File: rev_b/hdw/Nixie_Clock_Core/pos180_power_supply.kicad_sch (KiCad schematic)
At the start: 27 parts, among them Q601 IRFL214, U1301 TLV6700, U601 LT3757

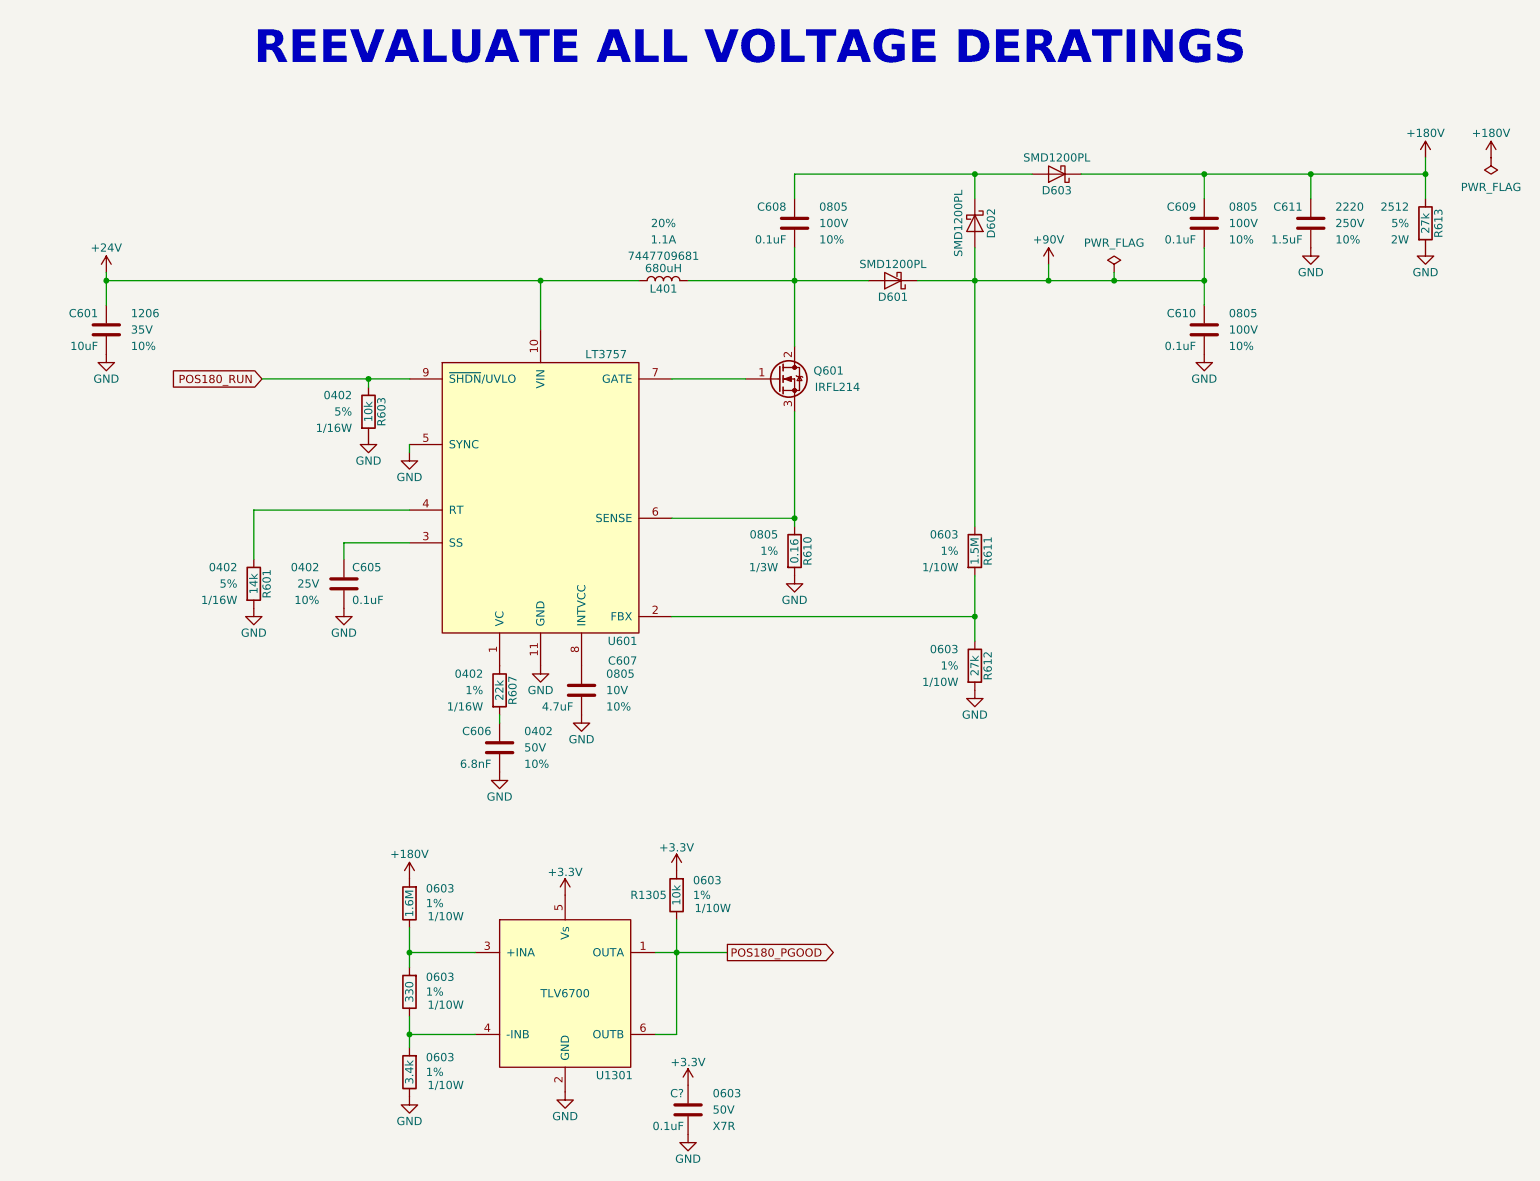
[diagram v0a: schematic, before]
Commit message: lots of rev B control board schematic progress
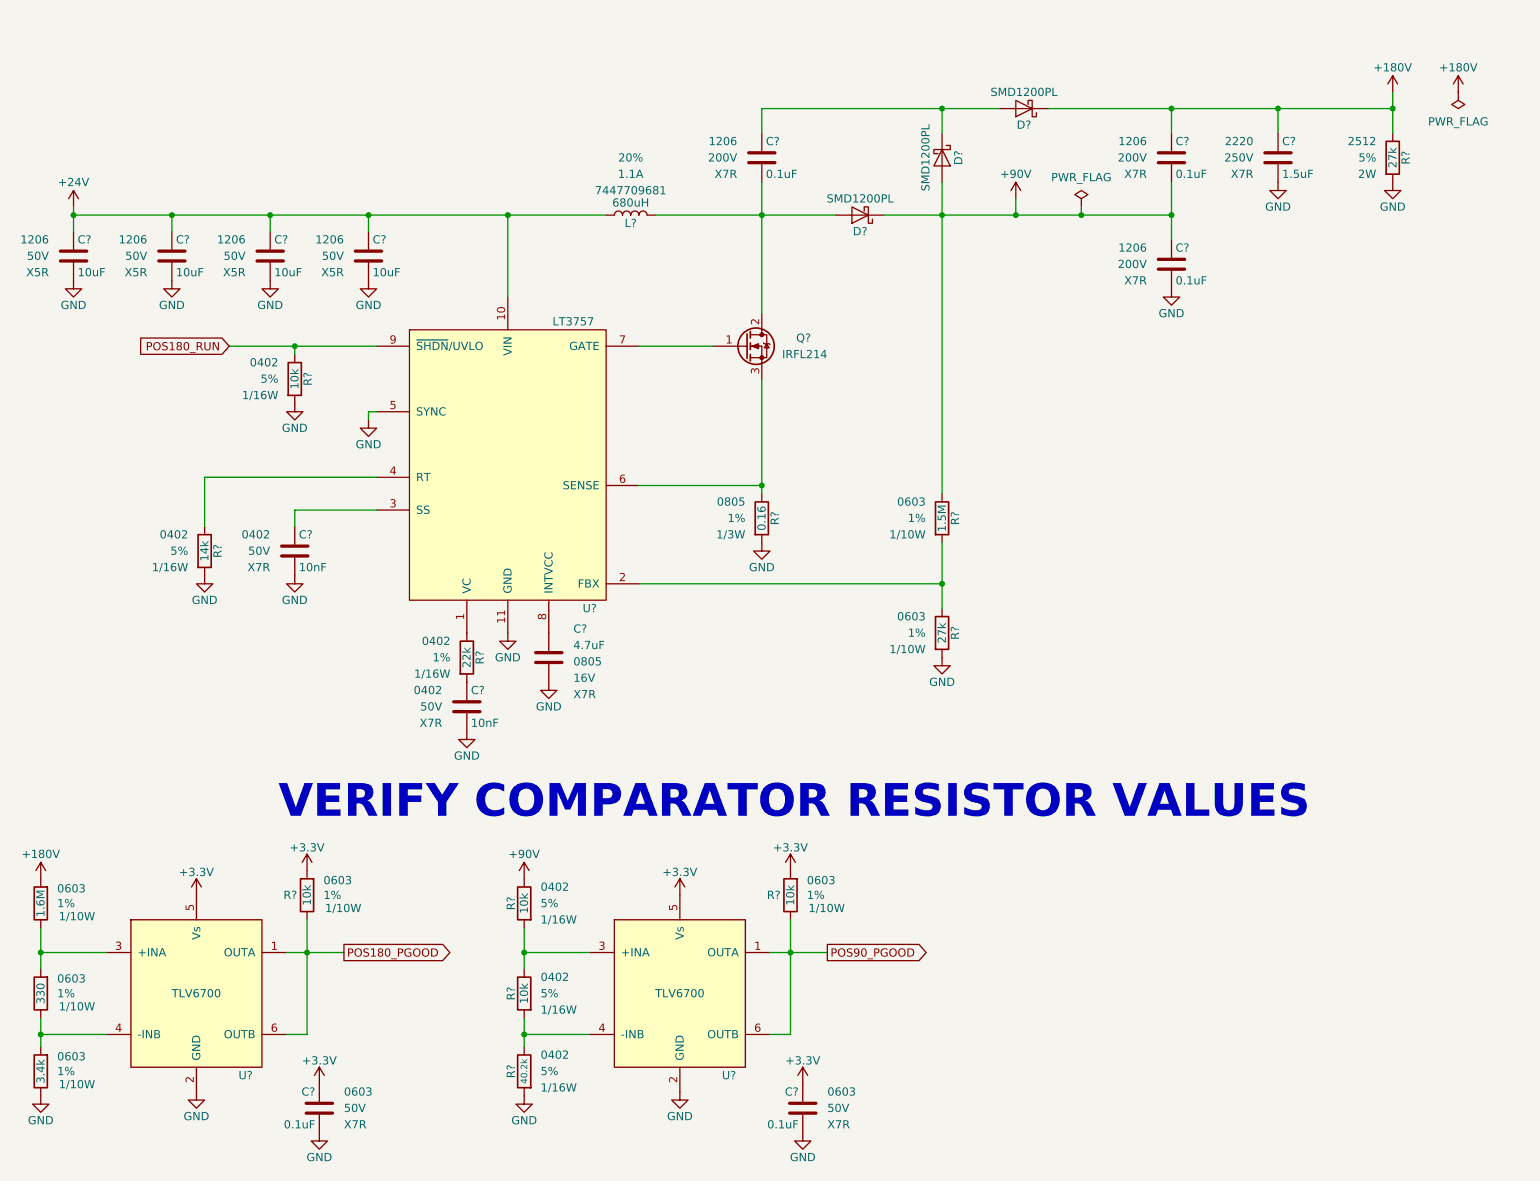
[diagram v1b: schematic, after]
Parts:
- removed C601: 10uF, Capacitors_SMD:C_1206, symbol Nixie-Clock-rescue:C
- removed C605: 0.1uF, Capacitors_SMD:C_0402, symbol Nixie-Clock-rescue:C
- removed C606: 6.8nF, Capacitors_SMD:C_0402, symbol Nixie-Clock-rescue:C
- removed C607: 4.7uF, Capacitors_SMD:C_0805, symbol Nixie-Clock-rescue:C
- removed C608, C609, C610: 0.1uF, Capacitors_SMD:C_0805, symbol Nixie-Clock-rescue:C
- removed C611: 1.5uF, Capacitors_SMD:C_2220, symbol Nixie-Clock-rescue:C
- added C? (x4): 10uF, symbol Custom Library:C_Custom
- added C? (x2): 10nF, Capacitors_SMD:C_0402, symbol Custom_Library:C_Custom
- added C? (x3): 0.1uF, symbol Custom Library:C_Custom
- added C?: 1.5uF, symbol Custom Library:C_Custom
- added C?: 4.7uF, Capacitors_SMD:C_0805, symbol Custom_Library:C_Custom
- added C?: 0.1uF, Capacitors_SMD:C_0603, symbol Custom_Library:C_Custom
- added R? (x2): 10k, Resistors_SMD:R_0402, symbol Nixie-Clock-rescue:R
- added R?: 40.2k, Resistors_SMD:R_0402, symbol Nixie-Clock-rescue:R
- added R?: 10k, Resistors_SMD:R_0603, symbol Custom_Library:R_Custom
- added U?: TLV6700, Package_TO_SOT_SMD:SOT-23-6, symbol Custom_Library:TLV6700
- L?: renamed from L401; Digi-Key PN 541-1236-1-ND -> 732-1700-1-ND
- Q?: renamed from Q601; Digi-Key PN (none) -> IRFL214PBFCT-ND
- renumbered D603 to D?, D601 to D?, D602 to D?, R610 to R?, R611 to R?, R603 to R?, R1305 to R?, R1302 to R?, R1304 to R?, R1303 to R?, R601 to R?, R607 to R?, R612 to R?, R613 to R?, U601 to U?, U1301 to U?
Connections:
- net +180V: now also C?.1, C?.1, C?.1, C?.2, R?.1
- net +24V: now also C?.1, C?.1, C?.1, C?.1
- net +3.3V: now also C?.1, R?.1, U?.5 (Vs)
- net GND: now also C?.2, C?.2, C?.2, C?.2, C?.2, C?.2, C?.2, C?.2, C?.2, C?.2, R?.2, U?.2 (GND)
- net at U?.3 (SS): now also C?.1
- net at U?.8 (INTVCC): now also C?.1
- net at R?.2: now also C?.1
- net at D?.1 (K), D?.2 (A): now also C?.1
- net at D?.2 (A), L?.2, Q?.2 (D): now also C?.2
- new net: R?.1, R?.2, U?.3 (+INA)
- new net: R?.1, R?.2, U?.4 (-INB)
- new net POS90_PGOOD: R?.2, U?.1 (OUTA), U?.6 (OUTB)
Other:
- note added: "VERIFY COMPARATOR RESISTOR VALUES"
- note removed: "REEVALUATE ALL VOLTAGE DERATINGS"
- moved on the sheet: C?, D?, L?, Q?, R?, U?
